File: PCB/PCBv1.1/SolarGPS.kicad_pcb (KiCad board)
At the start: 2 copper layers, 75 x 27 mm, 56 parts, among them J1 Conn_01x10_Female, J2 Solar1+, J3 GND, J4 Conn_02x03_Odd_Even, J5 Solar2+, J6 GND, J7 Screw_Terminal_01x01, U1 STM32L011G3Ux, U2 MAX-M10Q, U5 BQ25505, U6 LIS3DH, U7 TPS63802, Y1 32.768

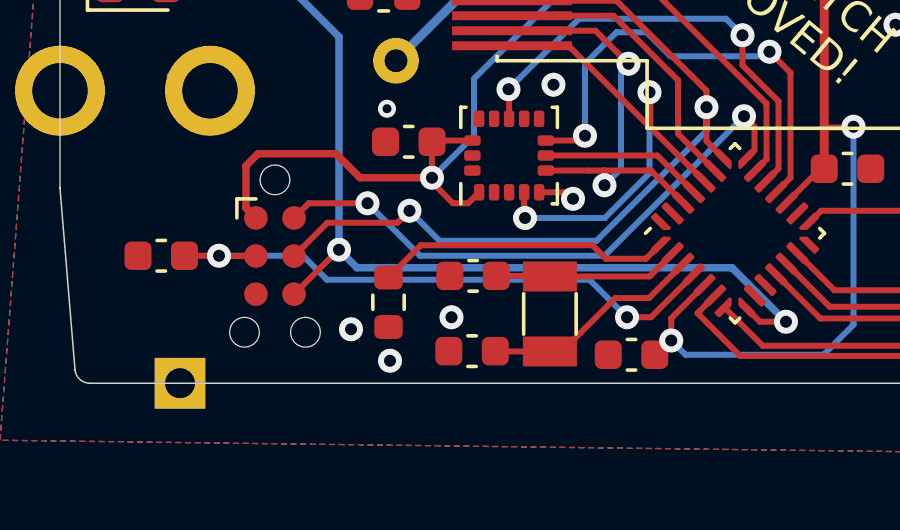
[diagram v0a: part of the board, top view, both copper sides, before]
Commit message: Tweak PCB
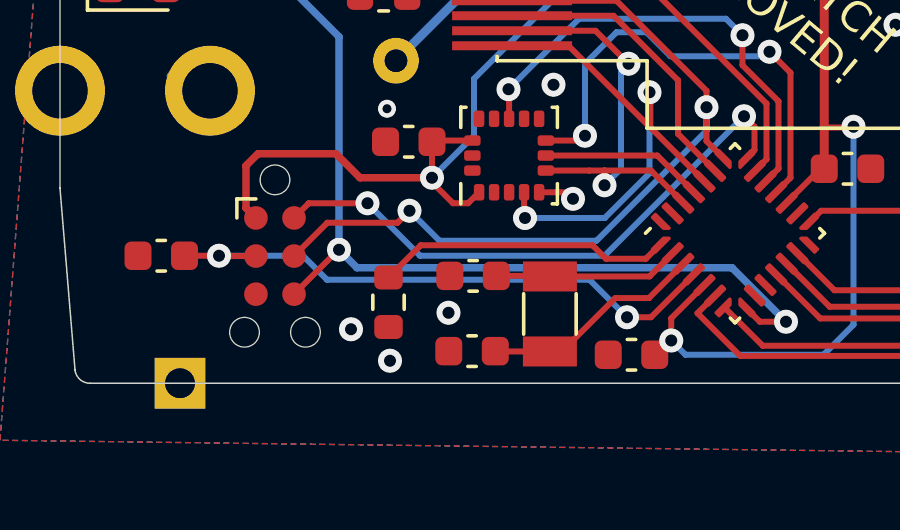
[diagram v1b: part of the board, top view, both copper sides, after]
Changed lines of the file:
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@@
   (via (at 87.75 60.65) (size 0.8) (drill 0.4) (layers "F.Cu" "B.Cu") (free) (net 1))
   (via (at 55.25 57.3) (size 0.6) (drill 0.3) (layers "F.Cu" "B.Cu") (free) (net 1))
-  (via (at 62.05 74.8) (size 0.8) (drill 0.4) (layers "F.Cu" "B.Cu") (free) (net 1))
+  (via (at 61.95 74.65) (size 0.8) (drill 0.4) (layers "F.Cu" "B.Cu") (free) (net 1))
   (via (at 57.8 63.35) (size 0.6) (drill 0.3) (layers "F.Cu" "B.Cu") (free) (net 1))
   (via (at 106.6 74.15) (size 0.8) (drill 0.4) (layers "F.Cu" "B.Cu") (free) (net 1))
